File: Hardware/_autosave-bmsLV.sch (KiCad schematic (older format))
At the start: 31 parts, among them J1 Conn_01x06_Male, J2 USB_B_Mini, J3 Conn_01x02_Female, J5 Conn_01x02_Female, K1 RM85V7, Q1 BSS138, SW1 SW_Push, U1 STM32F103C8Tx, Y1 Crystal

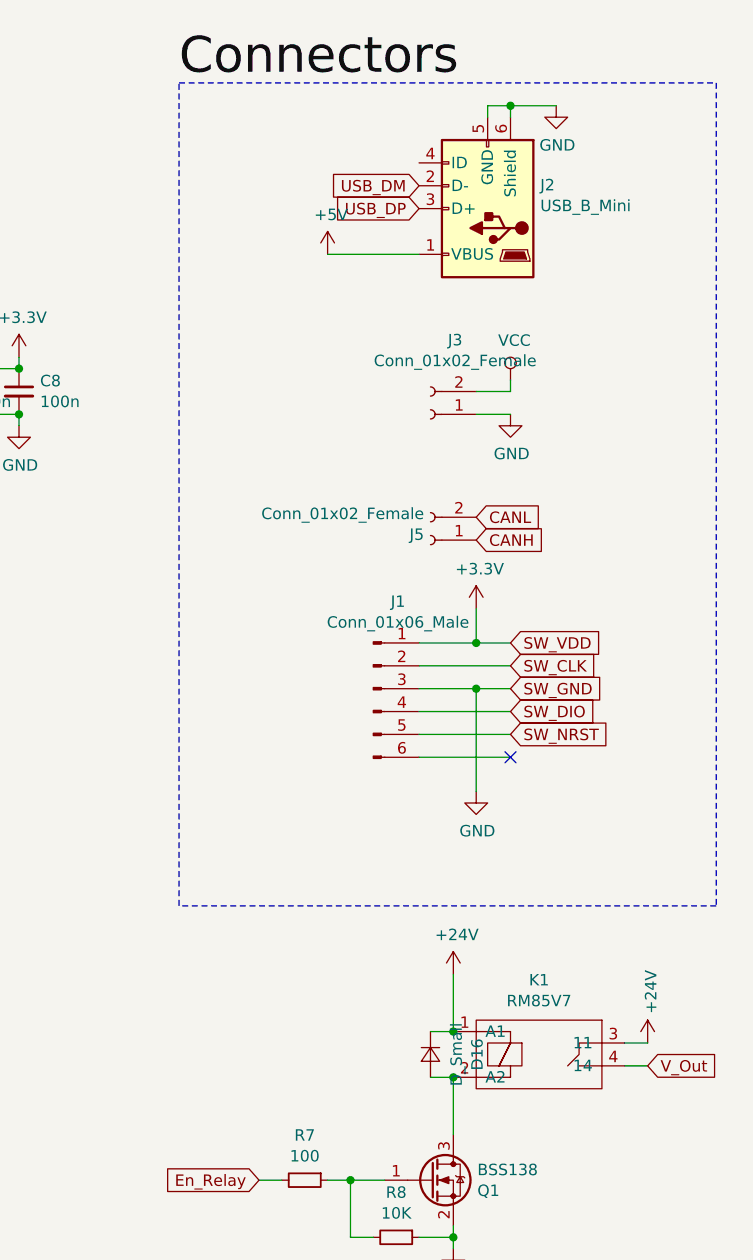
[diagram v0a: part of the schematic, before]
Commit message: Save before ZCO version
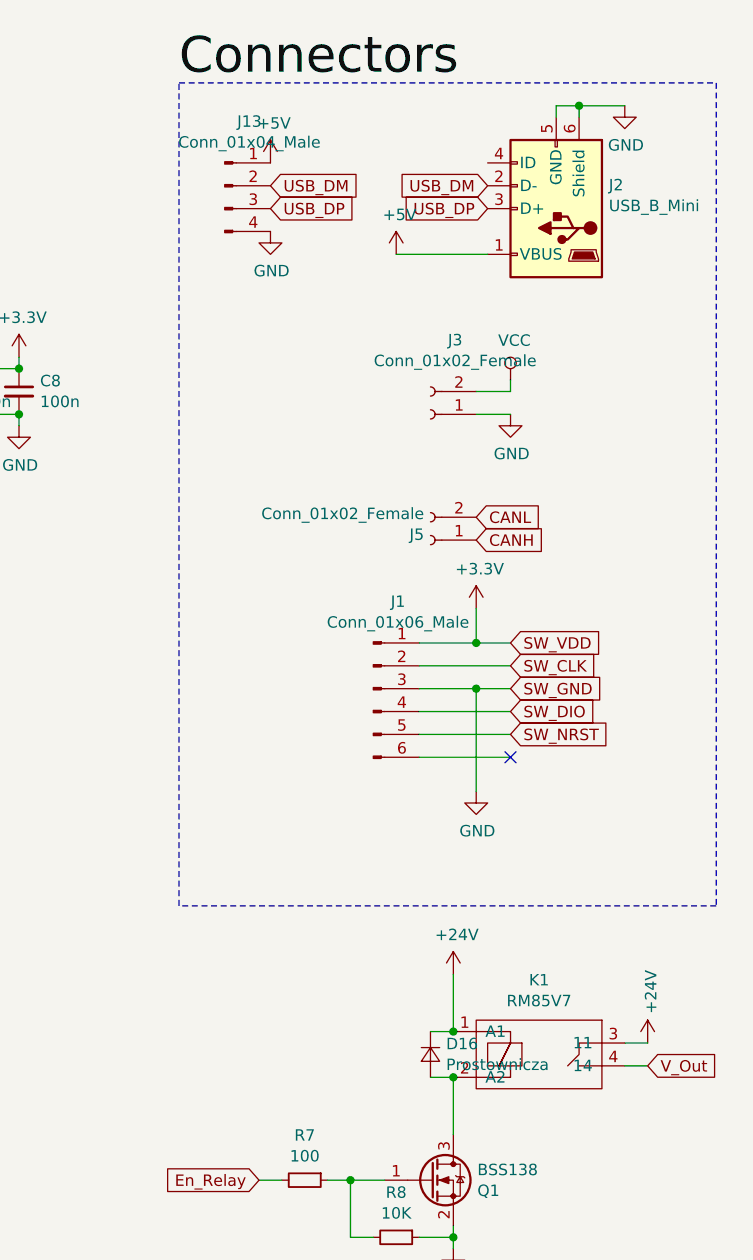
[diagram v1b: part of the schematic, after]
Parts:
- added J13: Conn_01x04_Male, Connector_PinHeader_2.54mm:PinHeader_1x04_P2.54mm_Vertical, symbol Connector:Conn_01x04_Male
- D16: value D_Small -> Prostownicza
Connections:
- net +5V: now also J13.1 (Pin_1)
- net GND: now also J13.4 (Pin_4)
- net USB_DM: now also J13.2 (Pin_2)
- net USB_DP: now also J13.3 (Pin_3)
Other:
- moved on the sheet: J2
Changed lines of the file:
@@
 L Connector:USB_B_Mini J2
 U 1 1 5FFA0FD0
-P 8150 1550
-F 0 "J2" H 7920 1447 50  0000 R CNN
-F 1 "USB_B_Mini" H 7920 1538 50  0000 R CNN
-F 2 "Connector_USB:USB_Micro-B_Molex_47346-0001" H 8300 1500 50  0001 C CNN
-F 3 "~" H 8300 1500 50  0001 C CNN
-	1    8150 1550
+P 8450 1550
+F 0 "J2" H 8220 1447 50  0000 R CNN
+F 1 "USB_B_Mini" H 8220 1538 50  0000 R CNN
+F 2 "Connector_USB:USB_Micro-B_Molex_47346-0001" H 8600 1500 50  0001 C CNN
+F 3 "~" H 8600 1500 50  0001 C CNN
+	1    8450 1550
 	-1   0    0    1
 $EndComp
@@
 L power:GND #PWR019
 U 1 1 5FFA2879
-P 8450 1100
-F 0 "#PWR019" H 8450 850 50  0001 C CNN
-F 1 "GND" H 8455 927 50  0000 C CNN
-F 2 "" H 8450 1100 50  0001 C CNN
-F 3 "" H 8450 1100 50  0001 C CNN
-	1    8450 1100
-	1    0    0    -1
-$EndComp
-Wire Wire Line
-	8150 1100 8150 1150
+P 8750 1100
+F 0 "#PWR019" H 8750 850 50  0001 C CNN
+F 1 "GND" H 8755 927 50  0000 C CNN
+F 2 "" H 8750 1100 50  0001 C CNN
+F 3 "" H 8750 1100 50  0001 C CNN
+	1    8750 1100
+	1    0    0    -1
+$EndComp
+Wire Wire Line
+	8450 1100 8450 1150
 $Comp
 L power:+5V #PWR014
 U 1 1 5FFAAF0D
-P 7450 1750
-F 0 "#PWR014" H 7450 1600 50  0001 C CNN
-F 1 "+5V" H 7465 1923 50  0000 C CNN
-F 2 "" H 7450 1750 50  0001 C CNN
-F 3 "" H 7450 1750 50  0001 C CNN
-	1    7450 1750
-	1    0    0    -1
-$EndComp
-Wire Wire Line
-	8150 1100 8250 1100
-Wire Wire Line
-	8250 1150 8250 1100
-Connection ~ 8250 1100
-Wire Wire Line
-	8250 1100 8450 1100
-Text GLabel 7850 1450 0    50   Input ~ 0
+P 7750 1750
+F 0 "#PWR014" H 7750 1600 50  0001 C CNN
+F 1 "+5V" H 7765 1923 50  0000 C CNN
+F 2 "" H 7750 1750 50  0001 C CNN
+F 3 "" H 7750 1750 50  0001 C CNN
+	1    7750 1750
+	1    0    0    -1
+$EndComp
+Wire Wire Line
+	8450 1100 8550 1100
+Wire Wire Line
+	8550 1150 8550 1100
+Connection ~ 8550 1100
+Wire Wire Line
+	8550 1100 8750 1100
+Text GLabel 8150 1450 0    50   Input ~ 0
 USB_DM
-Text GLabel 7850 1550 0    50   Input ~ 0
+Text GLabel 8150 1550 0    50   Input ~ 0
 USB_DP
 Wire Wire Line
-	7450 1750 7850 1750
+	7750 1750 8150 1750
 $Comp
 L power:+3.3V #PWR03
@@
 U 1 1 60308393
 P 7900 5250
-F 0 "D16" H 7900 5455 50  0000 C CNN
-F 1 "D_Small" H 7900 5364 50  0000 C CNN
+F 0 "D16" V 7854 5318 50  0000 L CNN
+F 1 "Prostownicza" V 7945 5318 50  0000 L CNN
 F 2 "Diode_SMD:D_SMB" V 7900 5250 50  0001 C CNN
 F 3 "~" V 7900 5250 50  0001 C CNN
@@
 	1    0    0    -1
 $EndComp
+$Comp
+L Connector:Conn_01x04_Male J13
+U 1 1 60342BDE
+P 7000 1450
+F 0 "J13" H 7108 1731 50  0000 C CNN
+F 1 "Conn_01x04_Male" H 7108 1640 50  0000 C CNN
+F 2 "Connector_PinHeader_2.54mm:PinHeader_1x04_P2.54mm_Vertical" H 7000 1450 50  0001 C CNN
+F 3 "~" H 7000 1450 50  0001 C CNN
+	1    7000 1450
+	1    0    0    -1
+$EndComp
+$Comp
+L power:+5V #PWR0104
+U 1 1 6034A78E
+P 7200 1350
+F 0 "#PWR0104" H 7200 1200 50  0001 C CNN
+F 1 "+5V" H 7215 1523 50  0000 C CNN
+F 2 "" H 7200 1350 50  0001 C CNN
+F 3 "" H 7200 1350 50  0001 C CNN
+	1    7200 1350
+	1    0    0    -1
+$EndComp
+Text GLabel 7200 1450 2    50   Input ~ 0
+USB_DM
+Text GLabel 7200 1550 2    50   Input ~ 0
+USB_DP
+$Comp
+L power:GND #PWR0105
+U 1 1 60352852
+P 7200 1650
+F 0 "#PWR0105" H 7200 1400 50  0001 C CNN
+F 1 "GND" H 7205 1477 50  0000 C CNN
+F 2 "" H 7200 1650 50  0001 C CNN
+F 3 "" H 7200 1650 50  0001 C CNN
+	1    7200 1650
+	1    0    0    -1
+$EndComp
